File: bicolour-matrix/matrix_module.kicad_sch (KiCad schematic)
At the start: 12 parts, among them U1 HT16K33A-28SSOP

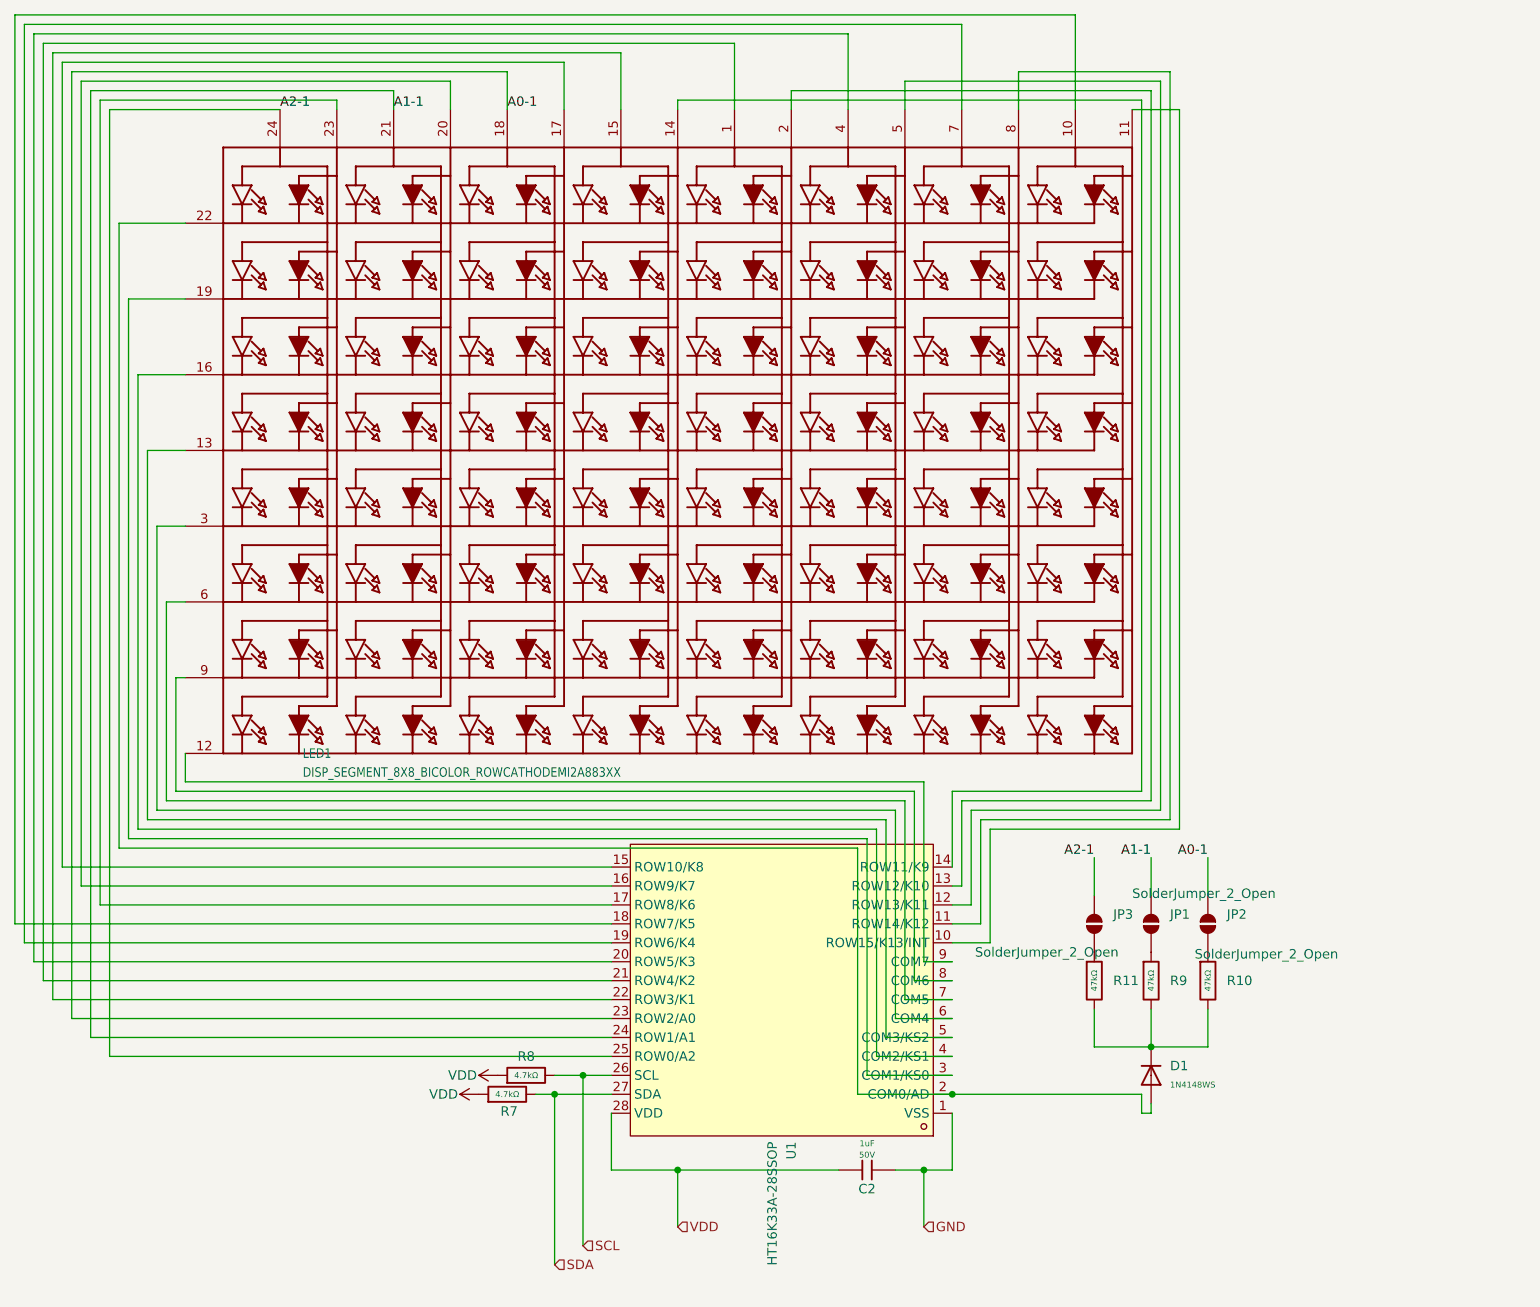
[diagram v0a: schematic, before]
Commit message: feat: all changes
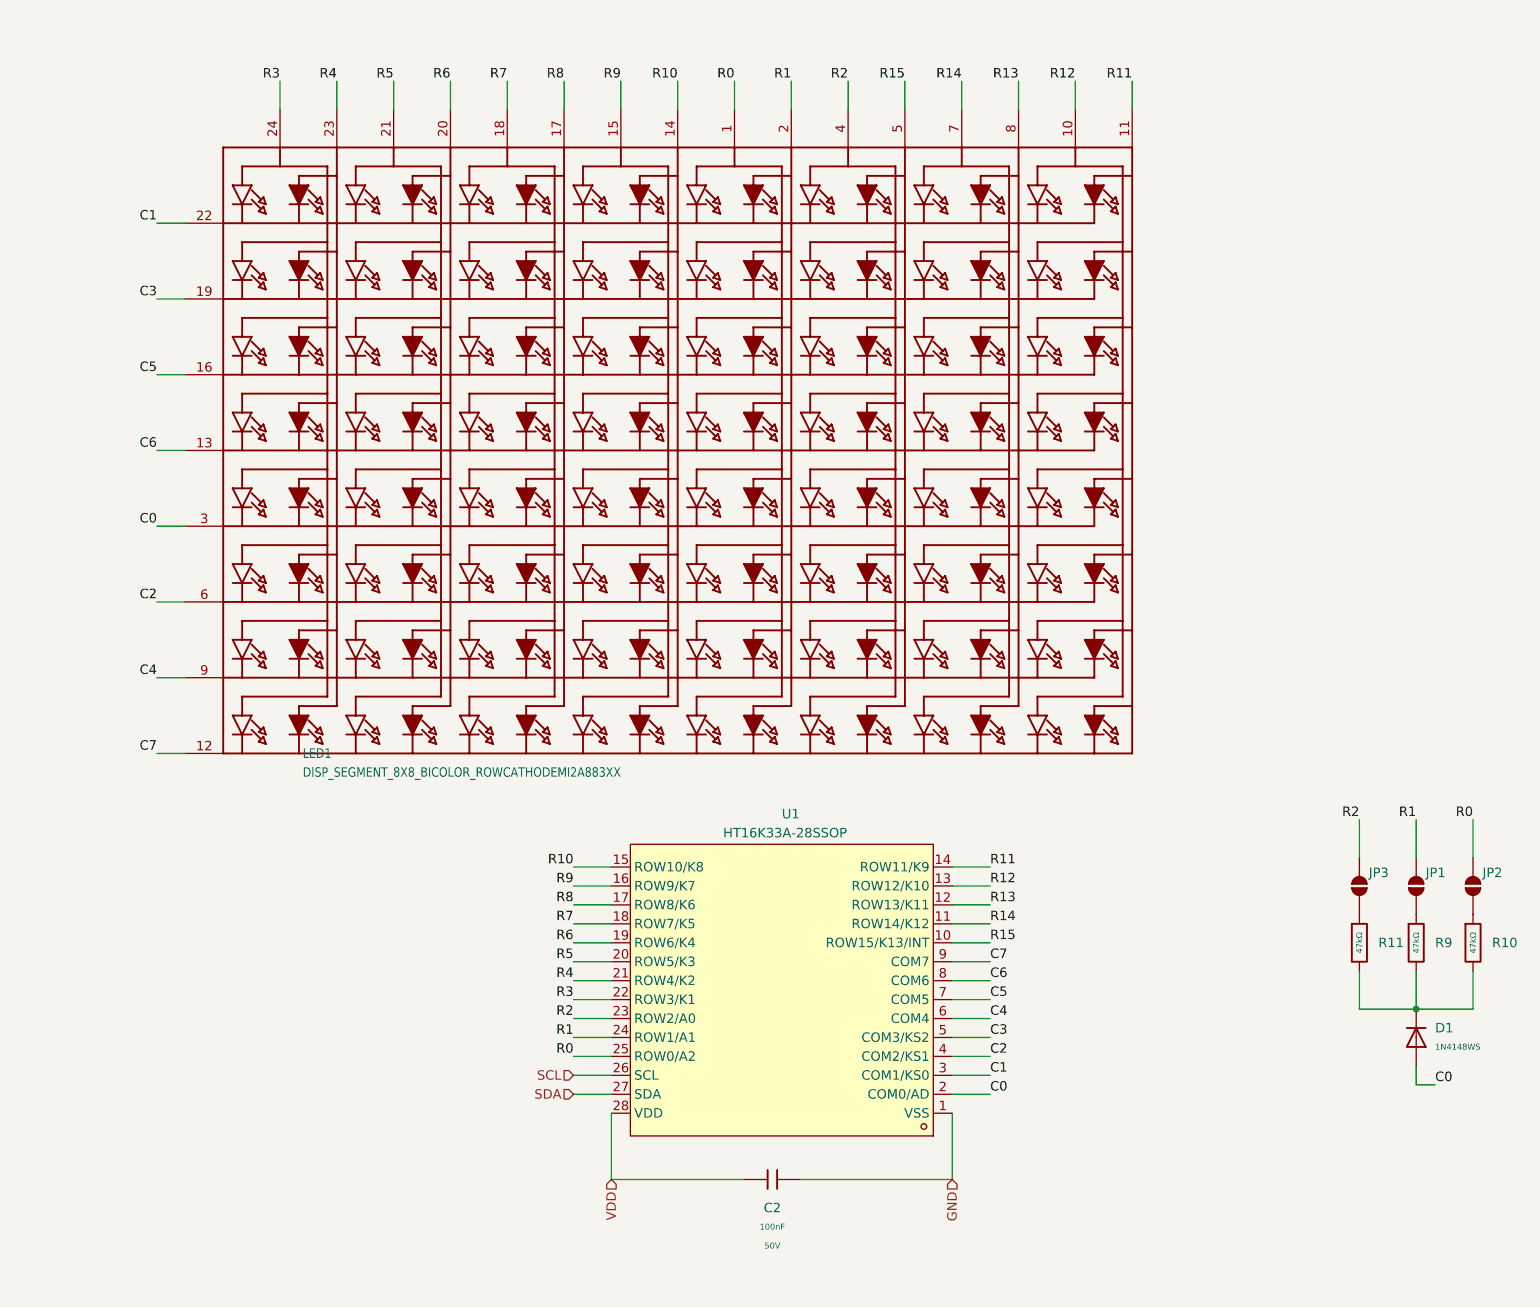
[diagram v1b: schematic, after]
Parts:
- removed C2: 1uF, PCM_JLCPCB:C_0603, symbol PCM_JLCPCB-Capacitors:0603,1uF
- removed R7, R8: 4.7kΩ, PCM_JLCPCB:R_0603, symbol PCM_JLCPCB-Resistors:0603,4.7kΩ
- added C2: 100nF, PCM_JLCPCB:C_0603, symbol PCM_JLCPCB-Capacitors:0603,100nF
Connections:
- net GND: now also C2.2
- net VDD: now also C2.1
- net R0: now reaches LED1.1 (A9)
- net R0: now also JP2.2 (B), U1.25 (ROW0/A2); no longer U1.21 (ROW4/K2)
- net R12: now reaches LED1.10 (A15)
- net R12: now also U1.13 (ROW12/K10); no longer U1.18 (ROW7/K5)
- net R11: now reaches LED1.11 (A16)
- net R11: now also U1.14 (ROW11/K9); no longer U1.10 (ROW15/K13/INT)
- net C7: now reaches LED1.12 (K8), U1.9 (COM7)
- net C3: now reaches U1.5 (COM3/KS2)
- net C3: now also LED1.19 (K2); no longer LED1.13 (K4)
- net R10: now reaches LED1.14 (A8)
- net R10: now also U1.15 (ROW10/K8); no longer U1.14 (ROW11/K9)
- net R3: now reaches U1.22 (ROW3/K1)
- net R3: now also LED1.24 (A1); no longer LED1.15 (A7)
- net C2: now reaches U1.4 (COM2/KS1)
- net C2: now also LED1.6 (K6); no longer LED1.16 (K3)
- net R8: now reaches LED1.17 (A6)
- net R8: now also U1.17 (ROW8/K6); no longer U1.15 (ROW10/K8)
- net C1: now reaches U1.3 (COM1/KS0)
- net C1: now also LED1.22 (K1); no longer LED1.19 (K2)
- net R1: now reaches LED1.2 (A10)
- net R1: now also JP1.2 (B), U1.24 (ROW1/A1); no longer U1.13 (ROW12/K10)
- net R6: now reaches LED1.20 (A4)
- net R6: now also U1.19 (ROW6/K4); no longer U1.16 (ROW9/K7)
- net C0: now reaches D1.2, U1.2 (COM0/AD)
- net C0: now also LED1.3 (K5); no longer LED1.22 (K1)
- net R4: now reaches LED1.23 (A2)
- net R4: now also U1.21 (ROW4/K2); no longer U1.17 (ROW8/K6)
- net C4: now reaches U1.6 (COM4)
- net C4: now also LED1.9 (K7); no longer LED1.3 (K5)
- net R2: now reaches LED1.4 (A11)
- net R2: now also JP3.2 (B), U1.23 (ROW2/A0); no longer U1.20 (ROW5/K3)
- net R13: now reaches U1.12 (ROW13/K11)
- net R13: now also LED1.8 (A14); no longer LED1.5 (A12)
- net C5: now reaches U1.7 (COM5)
- net C5: now also LED1.16 (K3); no longer LED1.6 (K6)
- net R14: now reaches LED1.7 (A13)
- net R14: now also U1.11 (ROW14/K12); no longer U1.19 (ROW6/K4)
- net C6: now reaches U1.8 (COM6)
- net C6: now also LED1.13 (K4); no longer LED1.9 (K7)
- removed net A0-1: JP2.2 (B), LED1.18 (A5), U1.23 (ROW2/A0)
- removed net A1-1: JP1.2 (B), LED1.21 (A3), U1.24 (ROW1/A1)
- removed net A2-1: JP3.2 (B), LED1.24 (A1), U1.25 (ROW0/A2)
- new net R15: LED1.5 (A12), U1.10 (ROW15/K13/INT)
- new net R5: LED1.21 (A3), U1.20 (ROW5/K3)
- new net R7: LED1.18 (A5), U1.18 (ROW7/K5)
- new net R9: LED1.15 (A7), U1.16 (ROW9/K7)
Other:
- moved on the sheet: D1, JP1, JP2, JP3, R10, R11, R9
